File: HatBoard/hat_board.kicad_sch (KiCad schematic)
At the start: 14 parts, among them J1 DF11 FC Connection, J13 DF11 FC Connection, J20 DF11 FC Connection, J21 DF11 FC Connection, U10 VEML7700, U12 DRV2605LDGS, U27 TMP112AIDRLR

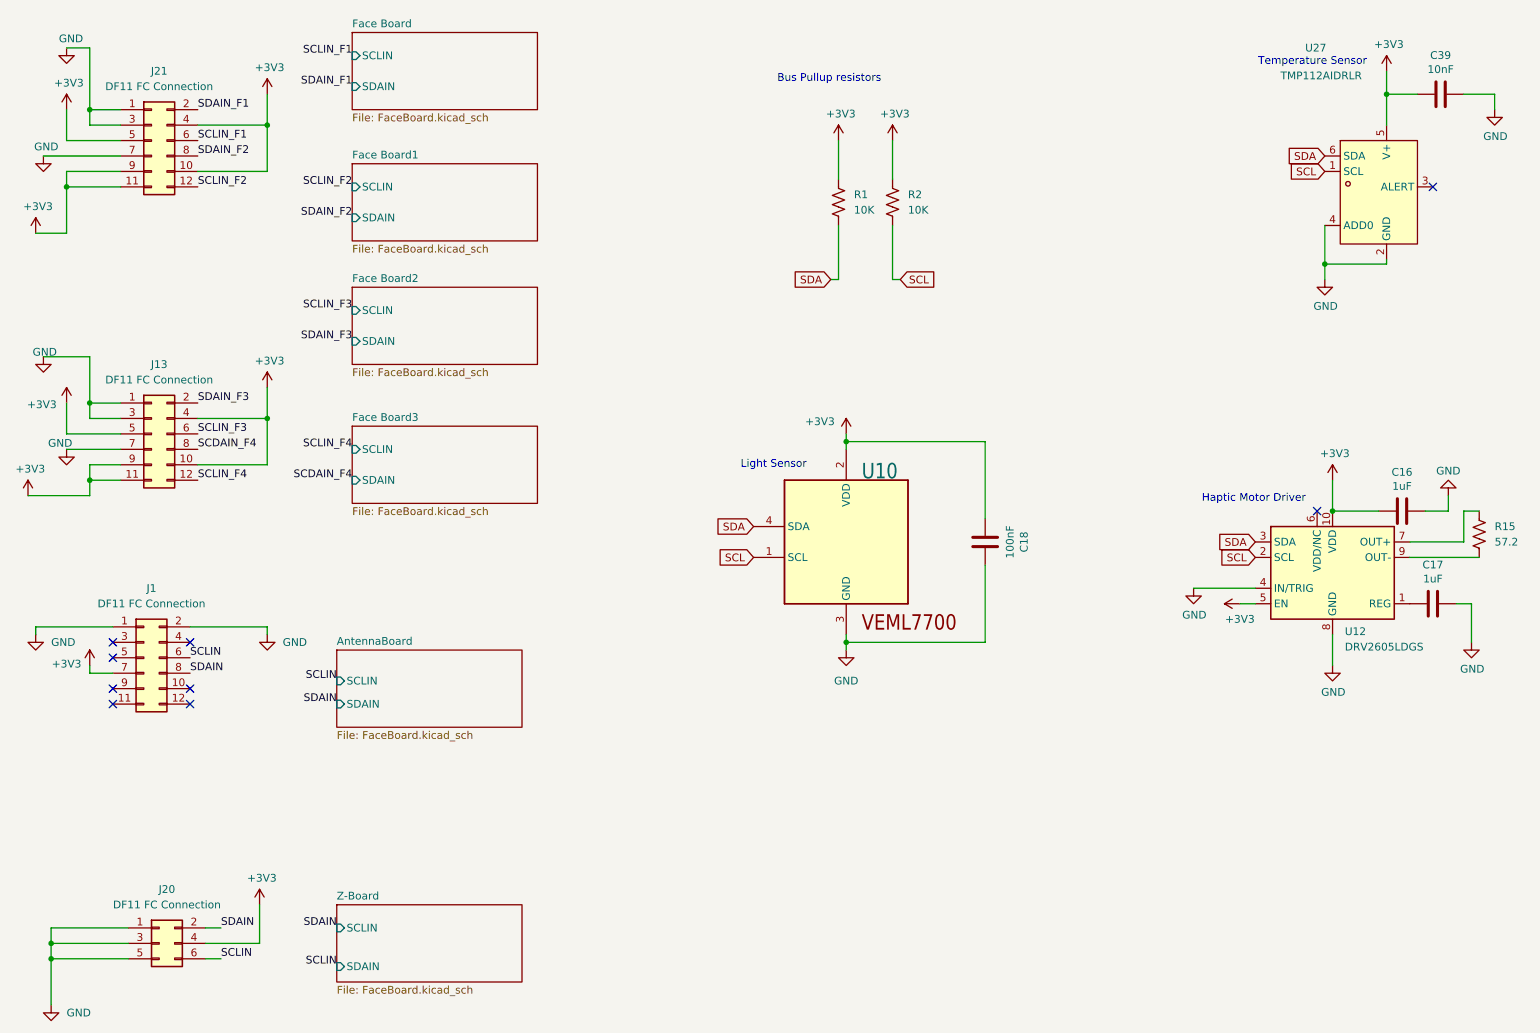
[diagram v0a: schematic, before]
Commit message: updated schematic
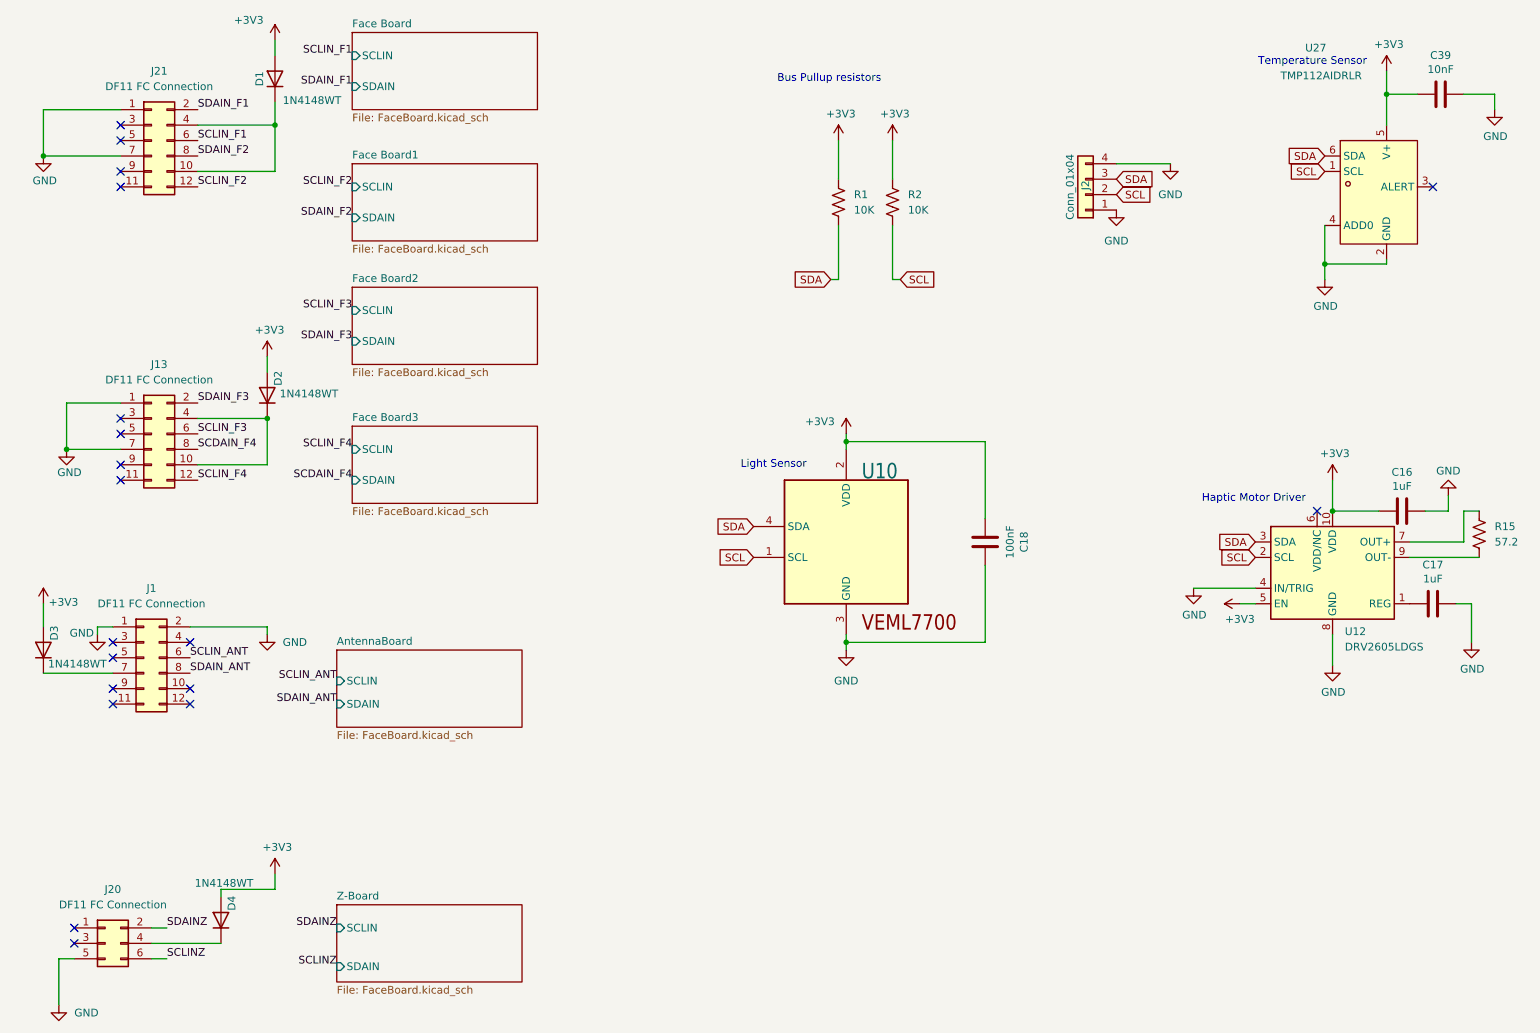
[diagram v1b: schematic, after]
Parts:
- added D1, D2, D3, D4: 1N4148WT, Diode_SMD:D_SOD-523, symbol Diode:1N4148WT
- added J2: Conn_01x04, Connector_PinHeader_2.00mm:PinHeader_1x04_P2.00mm_Vertical, symbol Connector_Generic:Conn_01x04
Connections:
- net +3V3: now also D1.2 (A), D2.2 (A), D3.2 (A), D4.2 (A); no longer J1.7 (Pin_7), J13.10 (Pin_10), J13.11 (Pin_11), J13.4 (Pin_4), J13.5 (Pin_5), J13.9 (Pin_9), J20.4 (Pin_4), J21.10 (Pin_10), J21.11 (Pin_11), J21.4 (Pin_4), J21.5 (Pin_5), J21.9 (Pin_9)
- net GND: now also J2.1 (Pin_1), J2.4 (Pin_4); no longer J13.3 (Pin_3), J20.1 (Pin_1), J20.3 (Pin_3), J21.3 (Pin_3)
- net SCL: now also J2.2 (Pin_2)
- net SDA: now also J2.3 (Pin_3)
- net SCLIN renamed SCLINZ
- net SCLINZ: no longer J1.6 (Pin_6)
- net SDAIN renamed SDAINZ
- net SDAINZ: no longer J1.8 (Pin_8)
- new net: D3.1 (K), J1.7 (Pin_7)
- new net: D2.1 (K), J13.10 (Pin_10), J13.4 (Pin_4)
- new net: D4.1 (K), J20.4 (Pin_4)
- new net: D1.1 (K), J21.10 (Pin_10), J21.4 (Pin_4)
- new net SCLIN_ANT: J1.6 (Pin_6)
- new net SDAIN_ANT: J1.8 (Pin_8)
- no-connect marks 9 -> 19
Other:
- moved on the sheet: J20
